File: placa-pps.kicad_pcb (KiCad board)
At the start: 2 copper layers, 61 x 88.9 mm, 10 parts, among them J1 CONN_01X06, J2 CONN_01X02, Q1 Q_NPN_BCE, Q2 Q_NPN_BCE, Q3 Q_NPN_BCE, U1 Huzzah-Feather, U3 KY-032

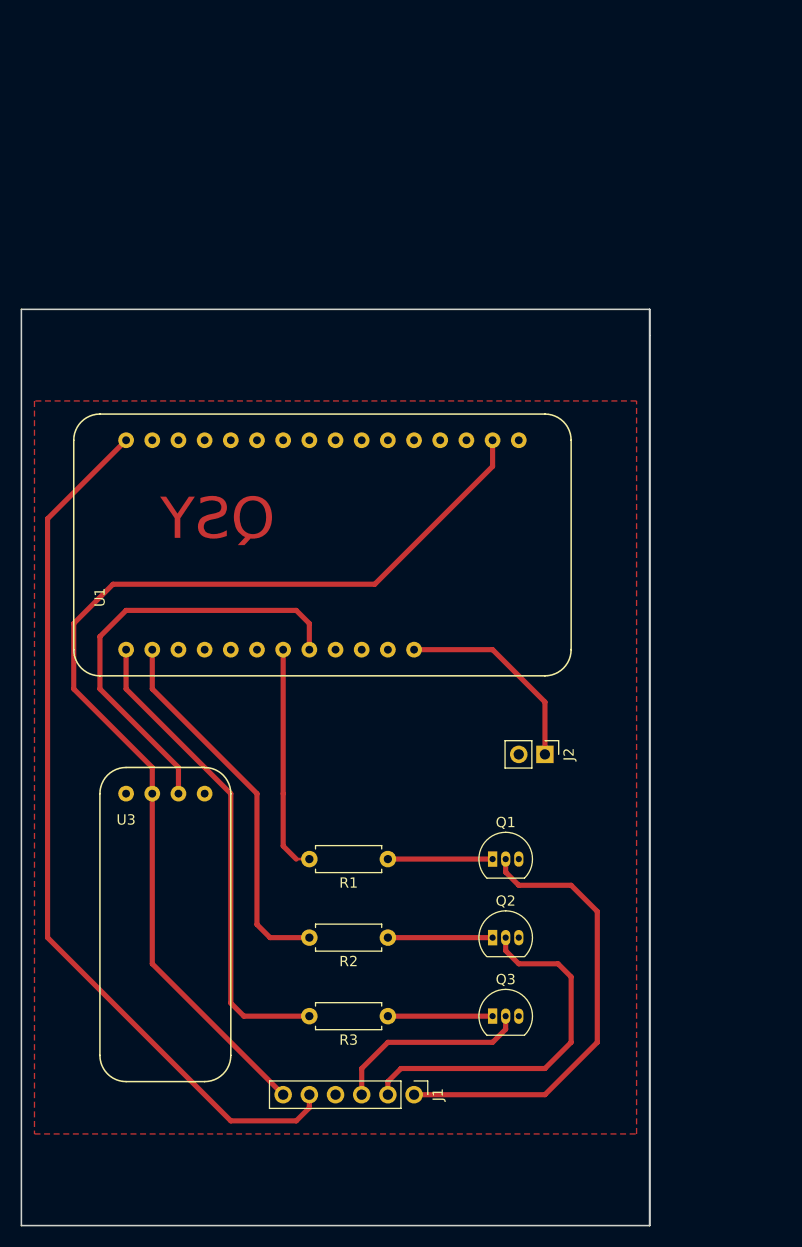
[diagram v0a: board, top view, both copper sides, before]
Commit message: Correcciones
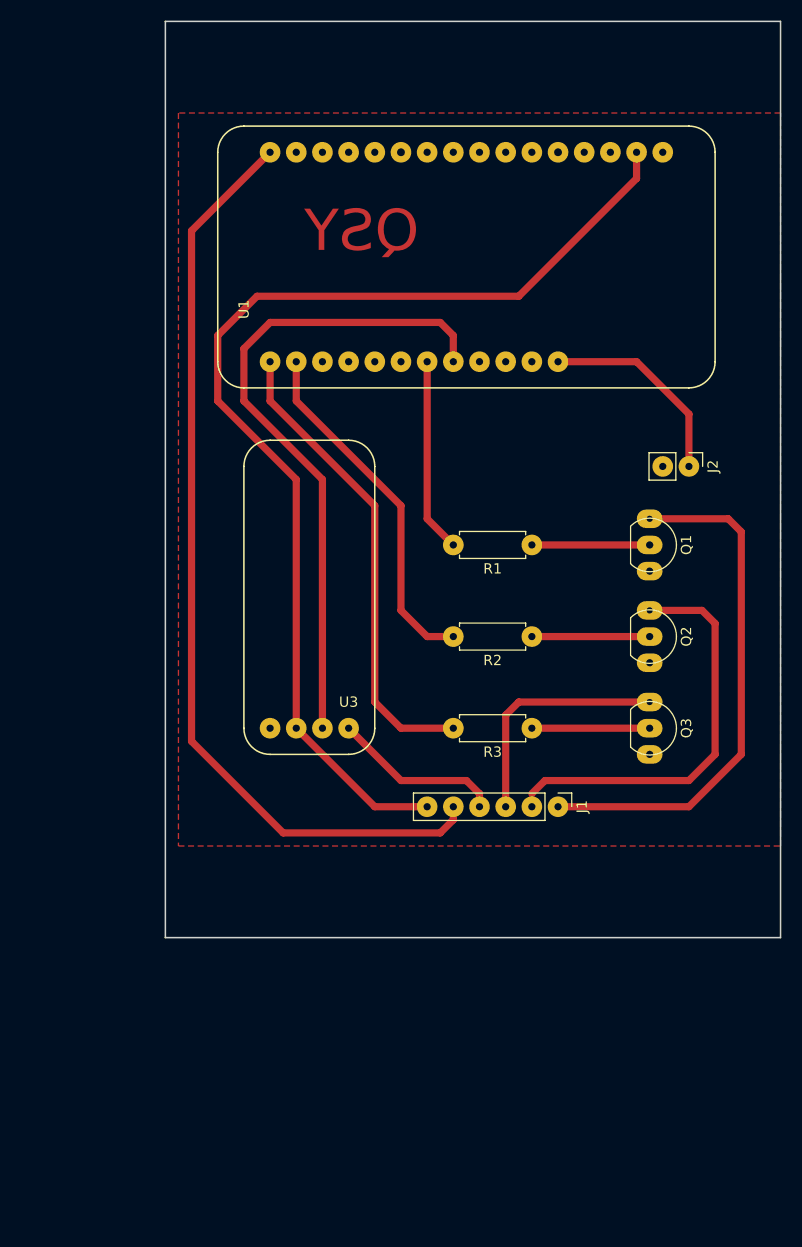
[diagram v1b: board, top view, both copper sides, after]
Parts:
- Q1, Q2, Q3: footprint TO_SOT_Packages_THT:TO-92_Inline_Narrow_Oval -> .pretty:TO-92_NPN
- moved Q1 35.2 mm to (101.6, 95.2), turned to 270 degrees
- moved Q2 34.1 mm to (101.6, 104.1), turned to 270 degrees
- moved R1 33.5 mm to (90.2, 96.5)
- moved Q3 32.9 mm to (101.6, 113.0), turned to 270 degrees
- moved R2 32.4 mm to (90.2, 105.4)
- moved J1 31.2 mm to (92.7, 121.9)
- moved R3 31.2 mm to (90.2, 114.3)
- moved J2 31.2 mm to (105.4, 88.9)
- moved U1 31.2 mm to (105.4, 71.1)
- moved U3 29.0 mm to (67.3, 104.1), turned to 0 degrees
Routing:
- net /SEN: track 42.8 -> 64.4 mm
- net GND: track 0.60 -> 16.6 mm
- net Net-(J1-Pad1): track 44.3 -> 50.9 mm
- net Net-(J1-Pad2): track 35.7 -> 40.2 mm
- net Net-(J1-Pad3): track 19.4 -> 23.4 mm
- net Net-(R1-Pad2): track 22.1 -> 18.8 mm
- net +3V3: track 103.6 -> 106.6 mm
- net /SW: track 88.5 -> 91.2 mm
- net Net-(R2-Pad2): track 36.5 -> 34.5 mm
- net Net-(Q3-Pad1): track 10.2 -> 11.4 mm
- net Net-(Q2-Pad1): track 10.2 -> 11.4 mm
- net Net-(Q1-Pad1): track 10.2 -> 11.4 mm
- net Net-(R3-Pad2): track 46.6 -> 45.9 mm
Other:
- board size 61 x 88.9 mm -> 59.7 x 88.9 mm
- net class Default: trace_width 0.5 -> 0.7
